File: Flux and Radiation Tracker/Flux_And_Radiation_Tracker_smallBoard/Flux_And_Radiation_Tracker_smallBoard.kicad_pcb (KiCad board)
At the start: 2 copper layers, 14 parts, among them J1 Conn_01x07, U1 LTR-390UV-01, U2 MMC5983MA

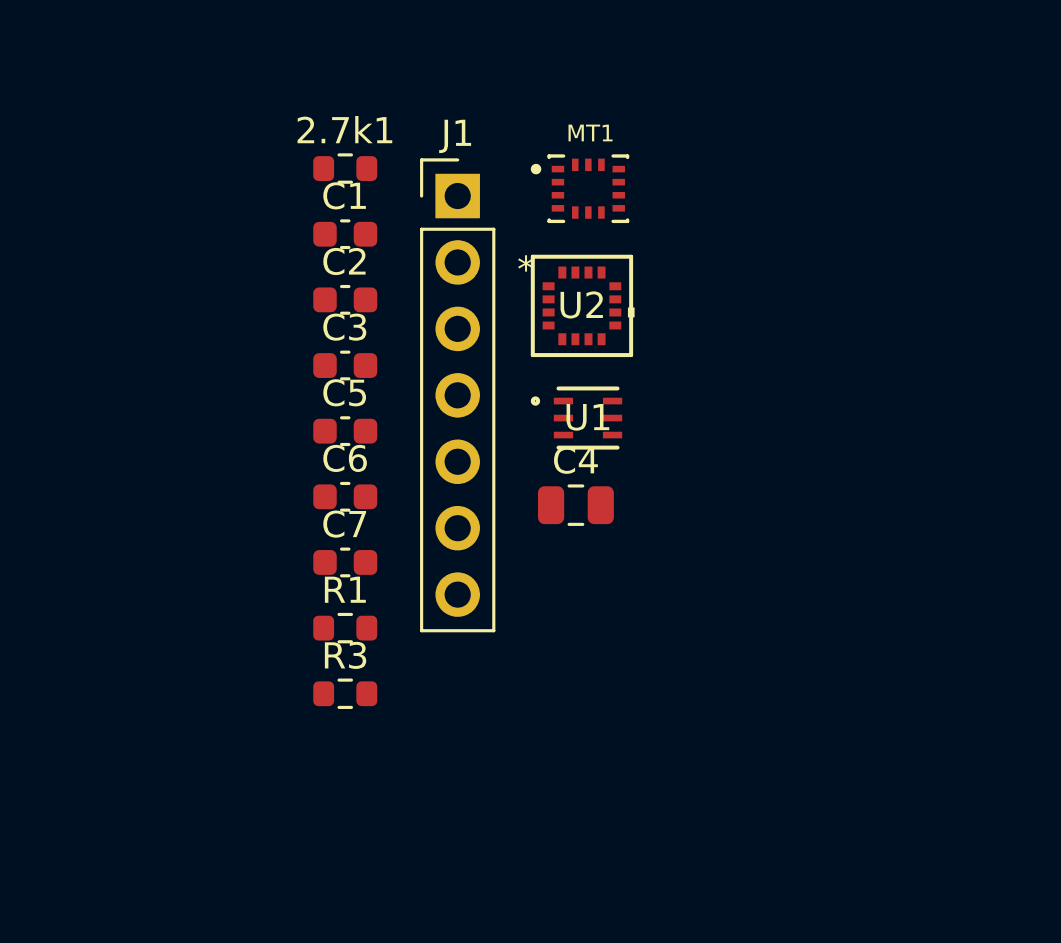
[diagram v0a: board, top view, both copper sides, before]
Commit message: Add files via upload
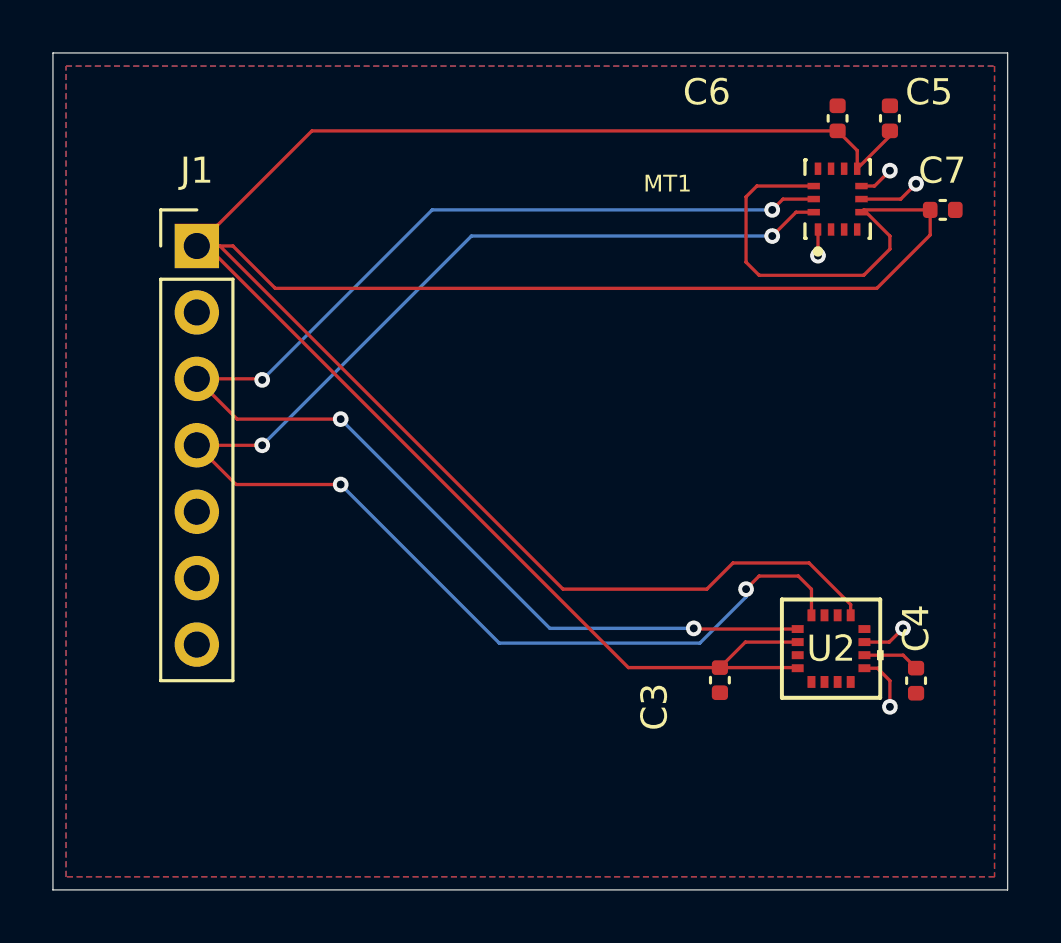
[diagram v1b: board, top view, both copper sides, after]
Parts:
- removed 2.7k1: R, Resistor_SMD:R_0603_1608Metric
- removed C1: 4.7u, Capacitor_SMD:C_0603_1608Metric
- removed C2: 0.1u, Capacitor_SMD:C_0603_1608Metric
- removed R1, R3: 2.7k, Resistor_SMD:R_0603_1608Metric
- removed U1: LTR-390UV-01, LTR-390UV:SMD6_LTR-390UV-01_LTO
- C3, C5, C6, C7: footprint Capacitor_SMD:C_0603_1608Metric -> Capacitor_SMD:C_0402_1005Metric
- C4: footprint Capacitor_SMD:C_0805_2012Metric -> Capacitor_SMD:C_0402_1005Metric
- moved C7 26.5 mm to (164.0, 85.5)
- moved C5 24.0 mm to (162.0, 82.0), turned to 90 degrees
- moved C6 23.7 mm to (160.0, 82.0), turned to 90 degrees
- moved C3 18.7 mm to (155.5, 103.5), turned to -90 degrees
- moved U2 16.2 mm to (159.8, 102.3)
- moved C4 14.6 mm to (163.0, 103.5), turned to -90 degrees
- moved J1 10.2 mm to (135.5, 86.9)
- moved MT1 9.54 mm to (160.0, 85.1), turned to 90 degrees
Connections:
- net /I2C_SCL renamed I2C_SCL
- net /I2C_SDA renamed I2C_SDA
- J1 pad 1: /3V3 -> +3.3V
- J1 pad 5: /LTR_INT -> unconnected-(J1-Pin_5-Pad5)
- J1 pad 6: /MAG_INT -> unconnected-(J1-Pin_6-Pad6)
- J1 pad 7: /LTR_INT -> unconnected-(J1-Pin_7-Pad7)
- MT1 pad 4: /ICM_INT1 -> unconnected-(MT1-INT1/INT-Pad4)
- MT1 pad 9: /ICM_INT2 -> unconnected-(MT1-INT2-Pad9)
- U2 pad 15: /MMC_INT -> unconnected-(U2-INT-Pad15)
- U2 pad 5: /MAG_SDO -> unconnected-(U2-SPI_SDO-Pad5)
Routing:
- net +3.3V: track 0.00 -> 141.5 mm
- net I2C_SDA: track 0.00 -> 56.4 mm, vias 0 -> 4
- net I2C_SCL: track 0.00 -> 53.4 mm, vias 0 -> 4
- net GND: track 0.00 -> 8.53 mm, vias 0 -> 5
- net Net-(U2-CAP): track 0.00 -> 2.18 mm
- added copper zone on B.Cu, net GND
- added copper zone on F.Cu, net GND
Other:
- board outline added: 36.5 x 32 mm
